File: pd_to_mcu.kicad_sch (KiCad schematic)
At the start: 10 parts

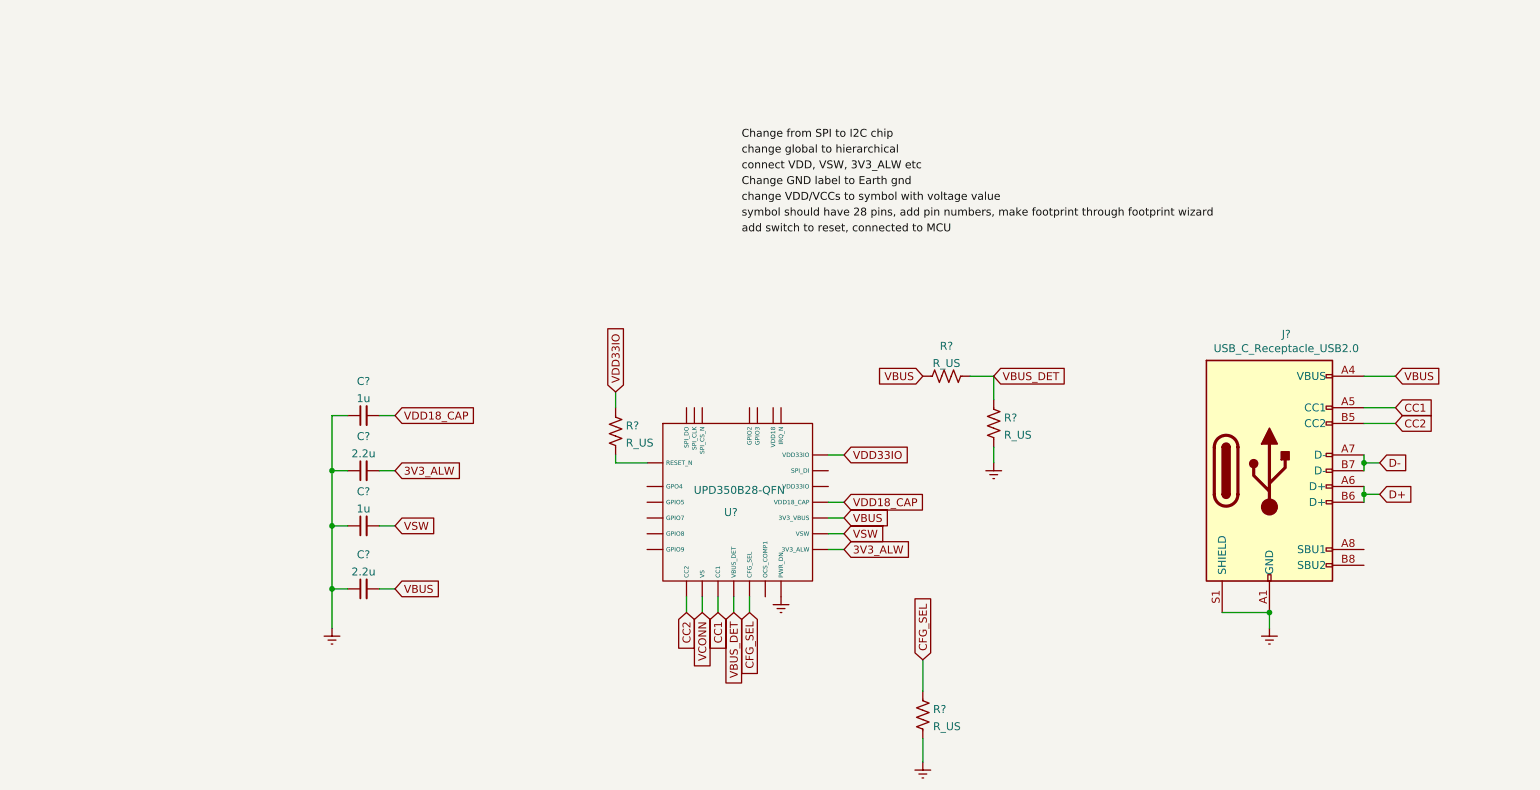
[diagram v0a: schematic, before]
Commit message: updated UPD
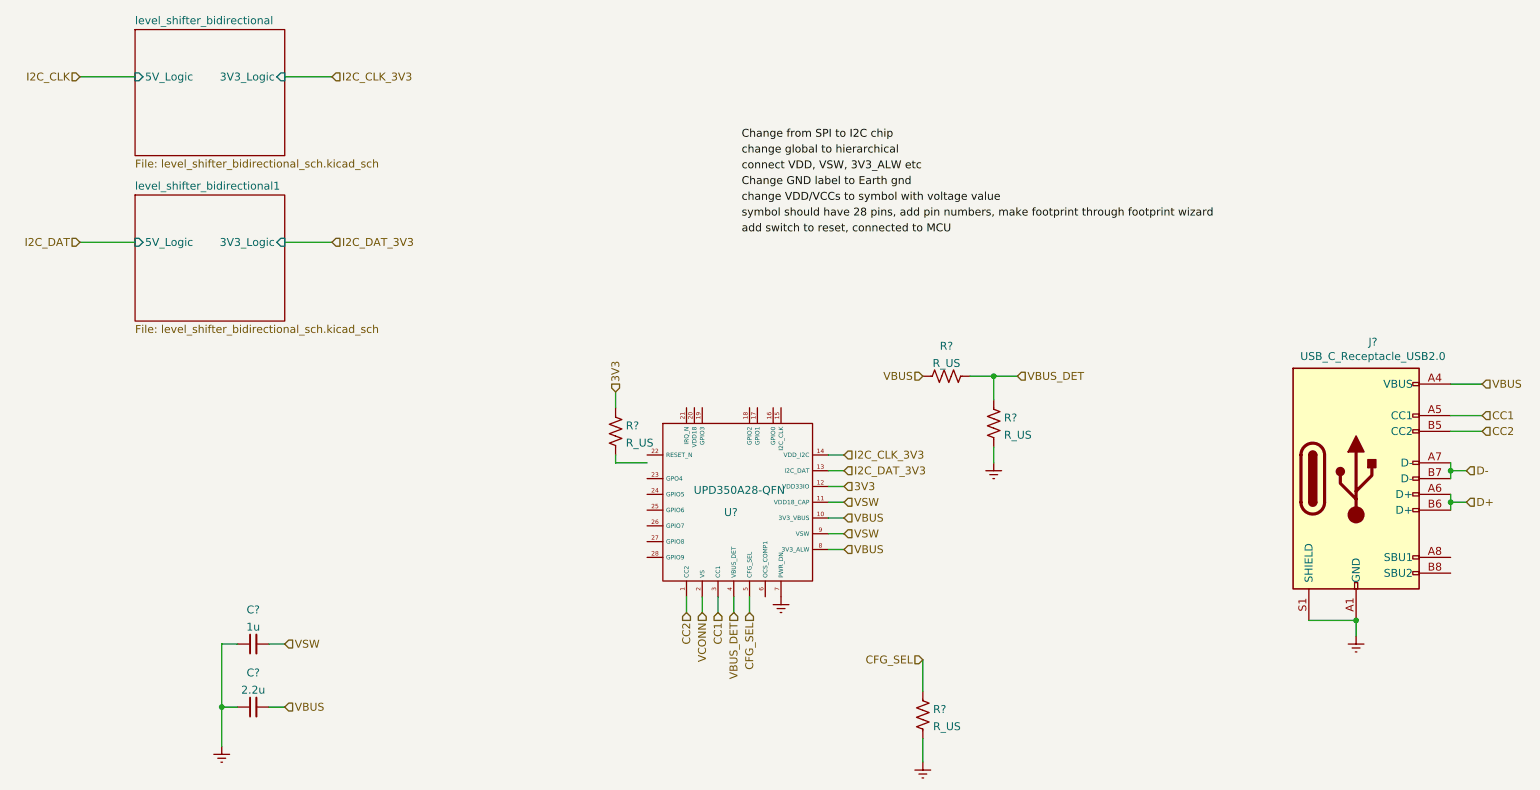
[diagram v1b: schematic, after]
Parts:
- removed C?: 2.2u, symbol Device:C_Small
- removed C?: 1u, symbol Device:C_Small
- U?: value UPD350B28-QFN -> UPD350A28-QFN
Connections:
- net CC1: now also U?.3 (CC1); no longer U?. (VSW)
- net CC2: now also U?.1 (CC2); no longer U?. (VSW)
- net CFG_SEL: now also U?.5 (CFG_SEL); no longer U?. (VSW)
- net Earth: now also U?.7 (PWR_DN); no longer U?. (VSW)
- net VBUS: now also U?.10 (3V3_VBUS), U?.8 (3V3_ALW); no longer U?. (VSW)
- net VBUS_DET: now also U?.4 (VBUS_DET); no longer U?. (VSW)
- net VCONN: now also U?.2 (VS); no longer U?. (VSW)
- net VSW: now also U?.11 (VDD18_CAP), U?.9 (VSW); no longer U?. (VSW)
- net at R?.2: no longer U?. (VSW)
- removed net 3V3_ALW: U?. (VSW)
- removed net VDD18_CAP: U?. (VSW)
- net VDD33IO renamed 3V3
- net 3V3: now also U?.12 (VDD33IO); no longer U?. (VSW)
- new net I2C_CLK_3V3: U?.14 (VDD_I2C)
- new net I2C_DAT_3V3: U?.13 (I2C_DAT)
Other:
- added sheet level_shifter_bidirectional (level_shifter_bidirectional_sch.kicad_sch)
- added sheet level_shifter_bidirectional1 (level_shifter_bidirectional_sch.kicad_sch)
- moved on the sheet: C?, J?
